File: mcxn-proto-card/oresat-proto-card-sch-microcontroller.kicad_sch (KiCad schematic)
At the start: 101 parts, among them U1 MCXN947VKLT, U8 TCAN330, Y2 24 MHz

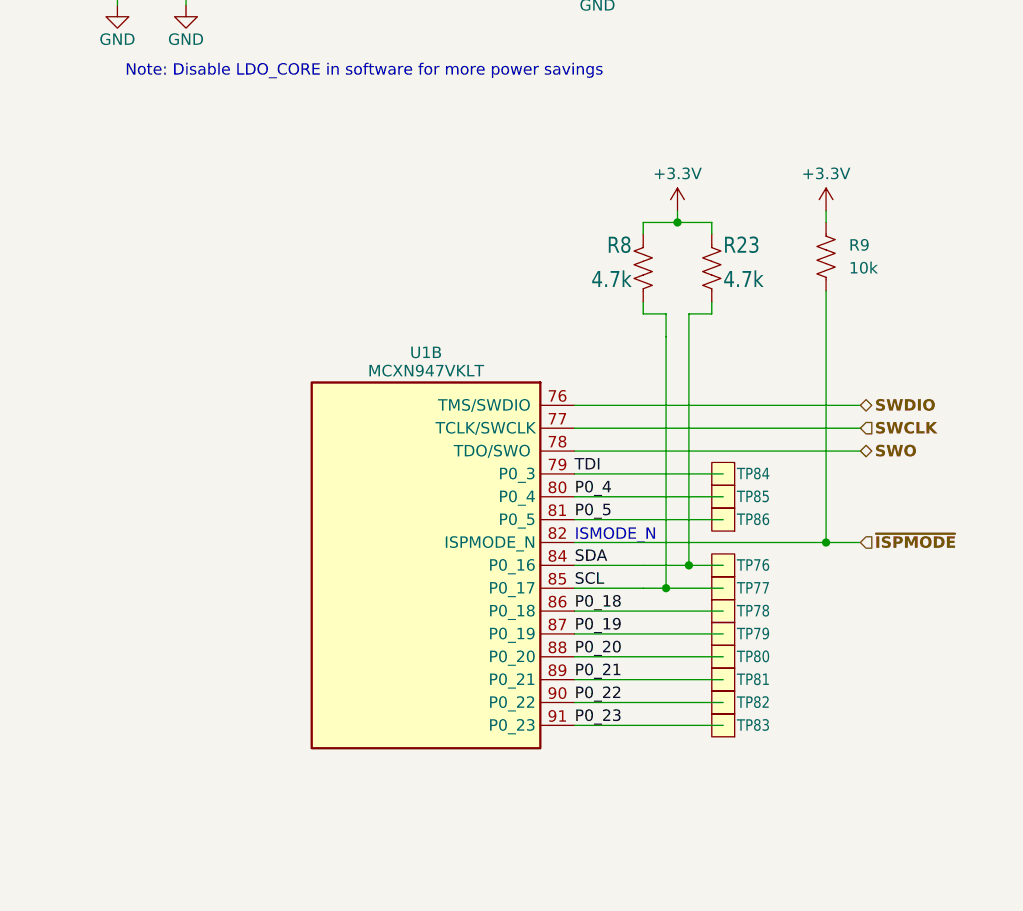
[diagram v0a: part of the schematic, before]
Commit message: Small cleanups for manufacturing
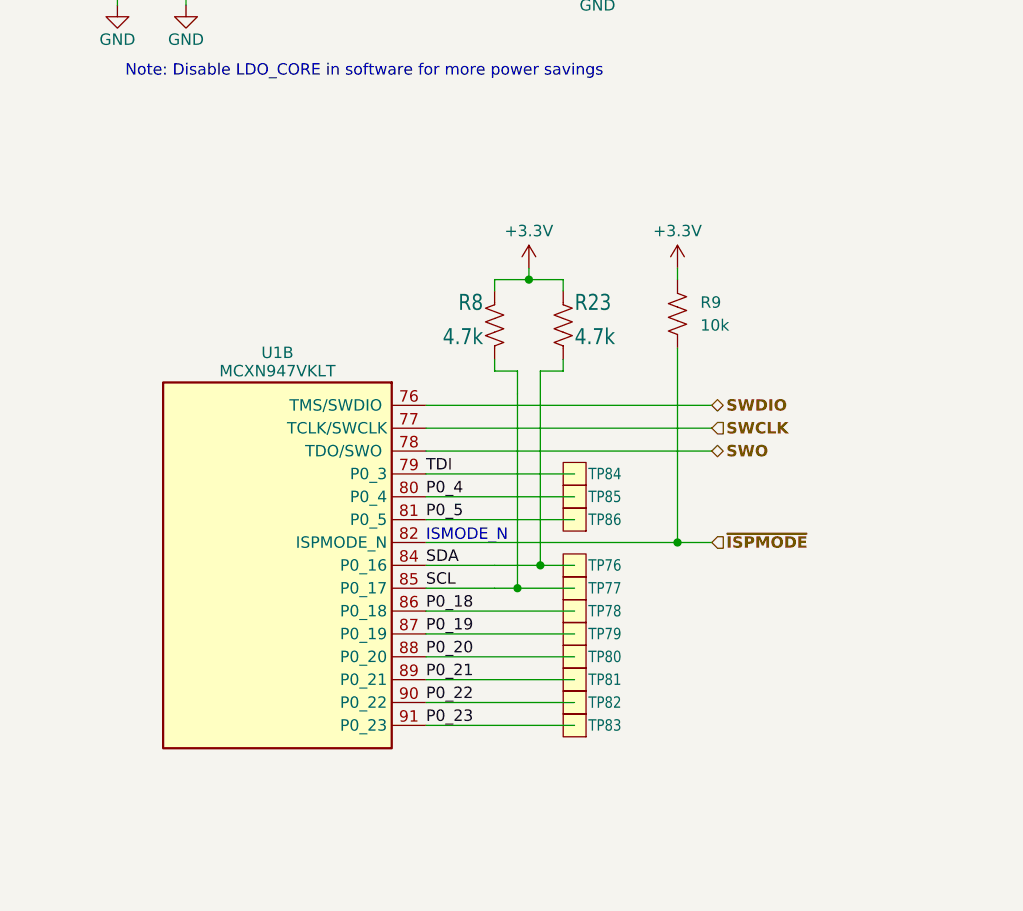
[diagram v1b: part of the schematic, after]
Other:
- moved on the sheet: R23, R8, R9, TP76, TP77, TP78, TP79, TP80, TP81, TP82, TP83, TP84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
